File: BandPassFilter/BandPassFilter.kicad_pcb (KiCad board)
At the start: 2 copper layers, 30.5 x 25.4 mm, 11 parts, among them J1 OUT, J2 INP

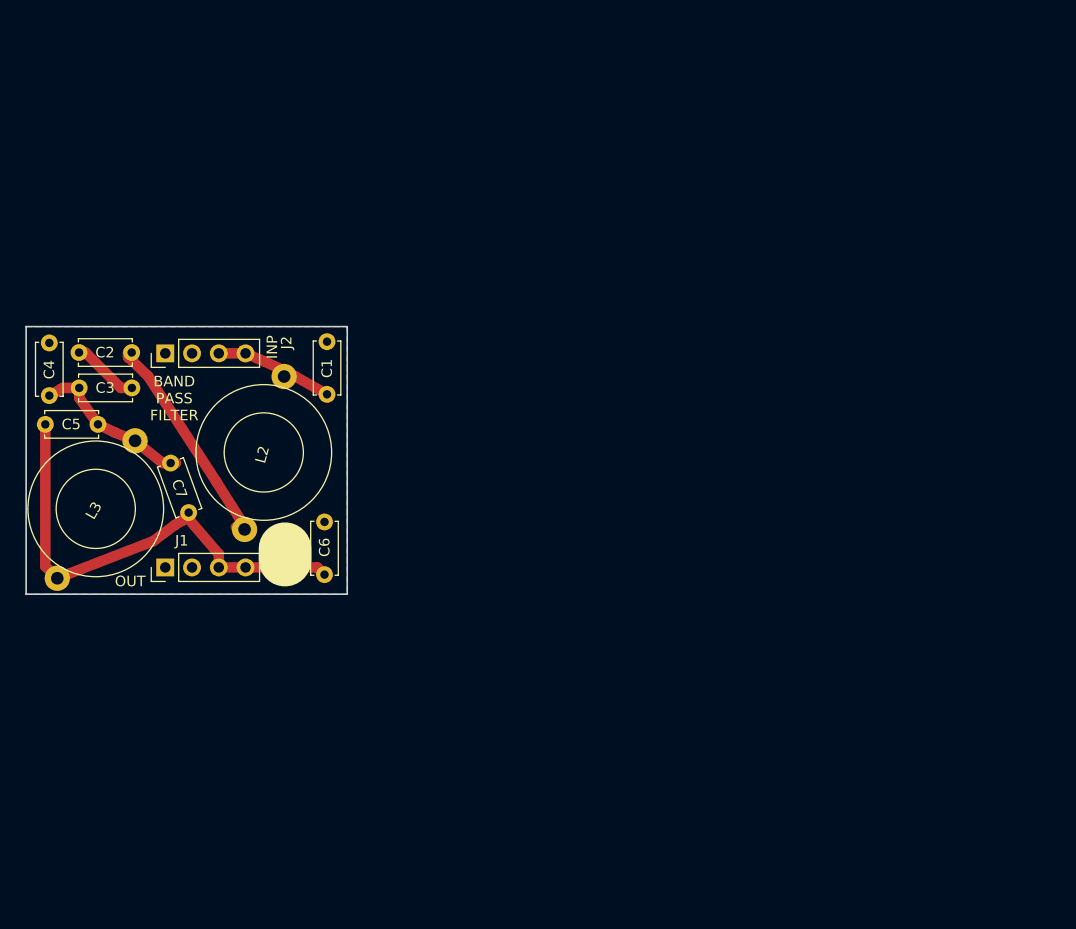
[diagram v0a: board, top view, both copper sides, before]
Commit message: BandPassFilter now has six filter boards on it
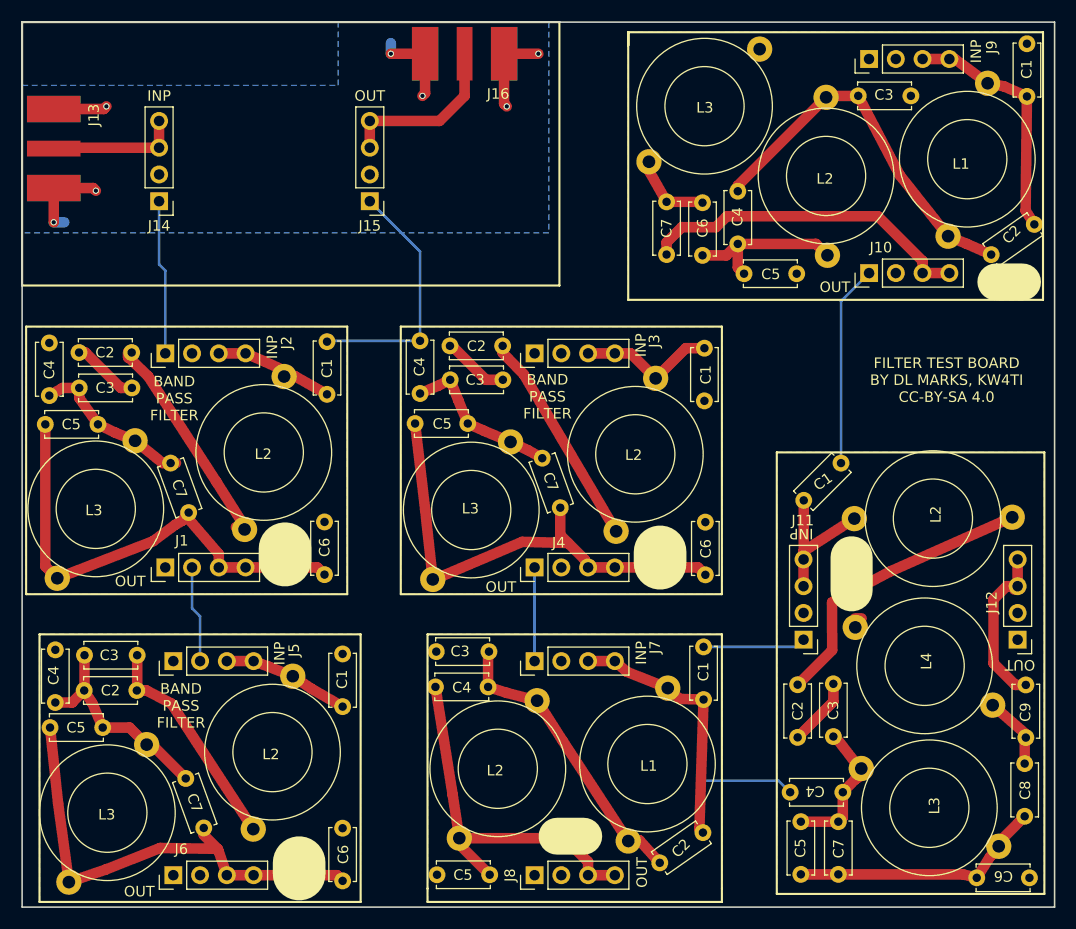
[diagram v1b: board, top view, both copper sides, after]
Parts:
- added C10: C3, Capacitors_THT:C_Disc_D5.0mm_W2.5mm_P5.00mm, F.Cu at (164.6, 94.0)
- added C11: C4, Capacitors_THT:C_Disc_D5.0mm_W2.5mm_P5.00mm, F.Cu at (156.8, 90.2)
- added C12: C7, Capacitors_THT:C_Disc_D5.0mm_W2.5mm_P5.00mm, F.Cu at (168.4, 101.4)
- added C13: C5, Capacitors_THT:C_Disc_D5.0mm_W2.5mm_P5.00mm, F.Cu at (161.3, 98.1)
- added C14: C6, Capacitors_THT:C_Disc_D5.0mm_W2.5mm_P5.00mm, F.Cu at (183.8, 107.5)
- added C15: C1, Capacitors_THT:C_Disc_D5.0mm_W2.5mm_P5.00mm, F.Cu at (149.4, 120.0)
- added C16: C3, Capacitors_THT:C_Disc_D5.0mm_W2.5mm_P5.00mm, F.Cu at (129.9, 120.1)
- added C17: C2, Capacitors_THT:C_Disc_D5.0mm_W2.5mm_P5.00mm, F.Cu at (129.9, 123.4)
- added C18: C4, Capacitors_THT:C_Disc_D5.0mm_W2.5mm_P5.00mm, F.Cu at (122.2, 119.6)
- added C19: C7, Capacitors_THT:C_Disc_D5.0mm_W2.5mm_P5.00mm, F.Cu at (134.5, 131.8)
- added C20: C5, Capacitors_THT:C_Disc_D5.0mm_W2.5mm_P5.00mm, F.Cu at (126.7, 127.0)
- added C21: C6, Capacitors_THT:C_Disc_D5.0mm_W2.5mm_P5.00mm, F.Cu at (149.4, 136.5)
- added C22: C1, Capacitors_THT:C_Disc_D5.0mm_W2.5mm_P5.00mm, F.Cu at (183.7, 119.3)
- added C23: C2, Capacitors_THT:C_Disc_D5.0mm_W2.5mm_P5.00mm, F.Cu at (183.6, 136.9)
- added C24: C3, Capacitors_THT:C_Disc_D5.0mm_W2.5mm_P5.00mm, F.Cu at (158.3, 119.8)
- added C25: C4, Capacitors_THT:C_Disc_D5.0mm_W2.5mm_P5.00mm, F.Cu at (163.2, 123.1)
- added C26: C5, Capacitors_THT:C_Disc_D5.0mm_W2.5mm_P5.00mm, F.Cu at (158.4, 140.9)
- added C27: C1, Capacitors_THT:C_Disc_D5.0mm_W2.5mm_P5.00mm, F.Cu at (214.4, 62.0)
- added C28: C2, Capacitors_THT:C_Disc_D5.0mm_W2.5mm_P5.00mm, F.Cu at (215.1, 79.2)
- added C29: C3, Capacitors_THT:C_Disc_D5.0mm_W2.5mm_P5.00mm, F.Cu at (203.4, 67.0)
- added C30: C4, Capacitors_THT:C_Disc_D5.0mm_W2.5mm_P5.00mm, F.Cu at (186.9, 76.0)
- added C31: C5, Capacitors_THT:C_Disc_D5.0mm_W2.5mm_P5.00mm, F.Cu at (192.5, 83.9)
- added C32: C6, Capacitors_THT:C_Disc_D5.0mm_W2.5mm_P5.00mm, F.Cu at (183.6, 82.1)
- added C33: C7, Capacitors_THT:C_Disc_D5.0mm_W2.5mm_P5.00mm, F.Cu at (180.2, 77.1)
- added C34: C1, Capacitors_THT:C_Disc_D5.0mm_W2.5mm_P5.00mm, F.Cu at (196.7, 101.9)
- added C35: C2, Capacitors_THT:C_Disc_D5.0mm_W2.5mm_P5.00mm, F.Cu at (192.6, 122.9)
- added C36: C3, Capacitors_THT:C_Disc_D5.0mm_W2.5mm_P5.00mm, F.Cu at (196.0, 122.8)
- added C37: C4, Capacitors_THT:C_Disc_D5.0mm_W2.5mm_P5.00mm, F.Cu at (191.9, 133.1)
- added C38: C7, Capacitors_THT:C_Disc_D5.0mm_W2.5mm_P5.00mm, F.Cu at (196.5, 135.9)
- added C39: C5, Capacitors_THT:C_Disc_D5.0mm_W2.5mm_P5.00mm, F.Cu at (192.9, 135.9)
- added C40: C6, Capacitors_THT:C_Disc_D5.0mm_W2.5mm_P5.00mm, F.Cu at (214.6, 141.2)
- added C41: C8, Capacitors_THT:C_Disc_D5.0mm_W2.5mm_P5.00mm, F.Cu at (214.2, 135.4)
- added C42: C9, Capacitors_THT:C_Disc_D5.0mm_W2.5mm_P5.00mm, F.Cu at (214.3, 127.9)
- added C8: C1, Capacitors_THT:C_Disc_D5.0mm_W2.5mm_P5.00mm, F.Cu at (183.8, 96.0)
- added C9: C2, Capacitors_THT:C_Disc_D5.0mm_W2.5mm_P5.00mm, F.Cu at (164.6, 90.7)
- added J10: OUT, Pin_Headers:Pin_Header_Straight_1x04_Pitch2.54mm, F.Cu at (199.4, 83.8)
- added J11: INP, Pin_Headers:Pin_Header_Straight_1x04_Pitch2.54mm, F.Cu at (193.2, 118.6)
- added J12: OUT, Pin_Headers:Pin_Header_Straight_1x04_Pitch2.54mm, F.Cu at (213.5, 118.6)
- added J13: Conn_Coaxial, BandPassFilter:Amphenol_RF_SMA_132289, F.Cu at (122.0, 72.0)
- added J14: INP, Pin_Headers:Pin_Header_Straight_1x04_Pitch2.54mm, F.Cu at (132.0, 77.0)
- added J15: OUT, Pin_Headers:Pin_Header_Straight_1x04_Pitch2.54mm, F.Cu at (152.0, 77.0)
- added J16: Conn_Coaxial, BandPassFilter:Amphenol_RF_SMA_132289, F.Cu at (161.0, 63.0)
- added J3: INP, Pin_Headers:Pin_Header_Straight_1x04_Pitch2.54mm, F.Cu at (167.6, 91.4)
- added J4: OUT, Pin_Headers:Pin_Header_Straight_1x04_Pitch2.54mm, F.Cu at (167.6, 111.8)
- added J5: INP, Pin_Headers:Pin_Header_Straight_1x04_Pitch2.54mm, F.Cu at (133.3, 120.7)
- added J6: OUT, Pin_Headers:Pin_Header_Straight_1x04_Pitch2.54mm, F.Cu at (133.3, 141.0)
- added J7: INP, Pin_Headers:Pin_Header_Straight_1x04_Pitch2.54mm, F.Cu at (167.6, 120.7)
- added J8: OUT, Pin_Headers:Pin_Header_Straight_1x04_Pitch2.54mm, F.Cu at (167.6, 141.0)
- added J9: INP, Pin_Headers:Pin_Header_Straight_1x04_Pitch2.54mm, F.Cu at (199.4, 63.5)
- added L1: L2, BandPassFilter:L_Toroid_Horizontal_D12.7mm_Compact, F.Cu at (179.8, 91.4)
- added L10: L2, BandPassFilter:L_Toroid_Horizontal_D12.7mm_Compact, F.Cu at (195.3, 64.6)
- added L11: L3, BandPassFilter:L_Toroid_Horizontal_D12.7mm_Compact, F.Cu at (176.7, 75.0)
- added L12: L2, BandPassFilter:L_Toroid_Horizontal_D12.7mm_Compact, F.Cu at (195.4, 107.1)
- added L13: L3, BandPassFilter:L_Toroid_Horizontal_D12.7mm_Compact, F.Cu at (196.4, 129.6)
- added L14: L4, BandPassFilter:L_Toroid_Horizontal_D12.7mm_Compact, F.Cu at (213.3, 126.1)
- added L4: L3, BandPassFilter:L_Toroid_Horizontal_D12.7mm_Compact, F.Cu at (166.6, 97.7)
- added L5: L2, BandPassFilter:L_Toroid_Horizontal_D12.7mm_Compact, F.Cu at (145.3, 119.6)
- added L6: L3, BandPassFilter:L_Toroid_Horizontal_D12.7mm_Compact, F.Cu at (132.1, 126.4)
- added L7: L1, BandPassFilter:L_Toroid_Horizontal_D12.7mm_Compact, F.Cu at (180.9, 120.8)
- added L8: L2, BandPassFilter:L_Toroid_Horizontal_D12.7mm_Compact, F.Cu at (169.2, 122.2)
- added L9: L1, BandPassFilter:L_Toroid_Horizontal_D12.7mm_Compact, F.Cu at (211.3, 63.4)
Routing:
- net GND: track 0.00 -> 125.6 mm, vias 0 -> 7
- net Net-(C12-Pad2): track 0.00 -> 46.6 mm
- net Net-(C19-Pad2): track 0.00 -> 45.9 mm
- net Net-(C25-Pad2): track 0.00 -> 36.2 mm
- net Net-(C28-Pad2): track 0.00 -> 35.8 mm
- net Net-(C33-Pad2): track 0.00 -> 31.9 mm
- net Net-(C35-Pad1): track 0.00 -> 28.1 mm
- net Net-(C23-Pad2): track 0.00 -> 28.0 mm
- net Net-(C22-Pad2): track 0.00 -> 24.8 mm
- net Net-(C38-Pad2): track 0.00 -> 24.3 mm
- net Net-(C27-Pad2): track 0.00 -> 23.3 mm
- net Net-(C16-Pad1): track 0.00 -> 21.2 mm
- net Net-(C9-Pad1): track 0.00 -> 20.8 mm
- net Net-(C16-Pad2): track 0.00 -> 20.7 mm
- net Net-(J15-Pad3): track 0.00 -> 16.5 mm
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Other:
- board size 30.5 x 25.4 mm -> 98 x 84 mm
- board text added: "C1"
- board text added: "C2"
- board text added: "C3"
- board text added: "C4"
- board text added: "C5"
- board text added: "C6"
- board text added: "C7"
- board text added: "C8"
- board text added: "C9"
- board text added: "FILTER TEST BOARD BY DL MARKS, KW4TI CC-BY-SA 4.0"
- board text added: "L1"
- board text added: "L2"
- board text added: "L3"
- board text added: "L4"
